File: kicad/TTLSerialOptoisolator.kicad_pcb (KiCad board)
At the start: 2 copper layers, 8 parts, among them P1 CONN_4, P2 CONN_4, U1 817C, U2 817C

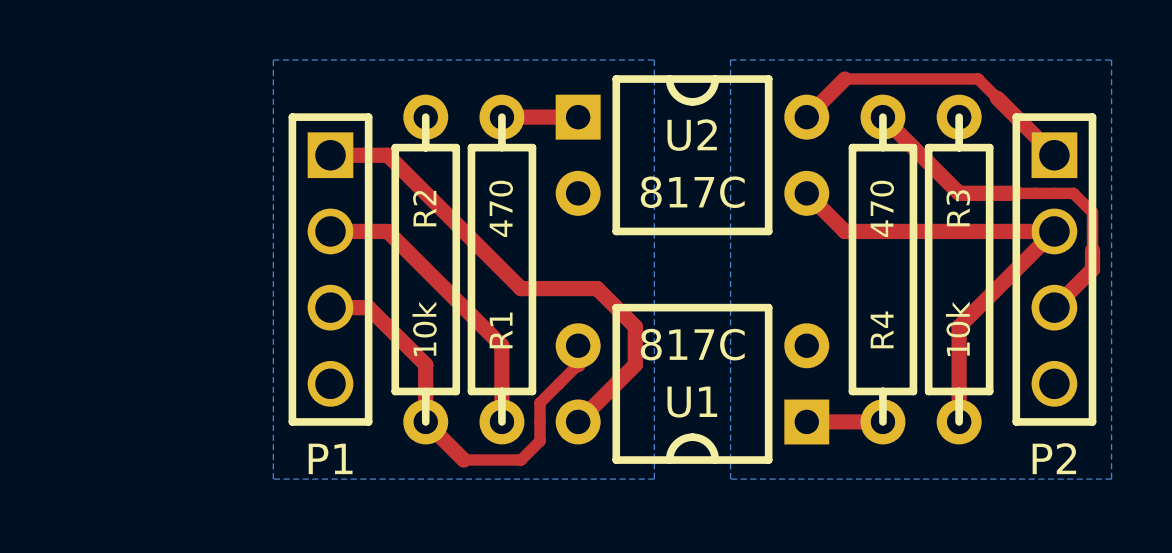
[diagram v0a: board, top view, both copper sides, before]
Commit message: iterating on board layout
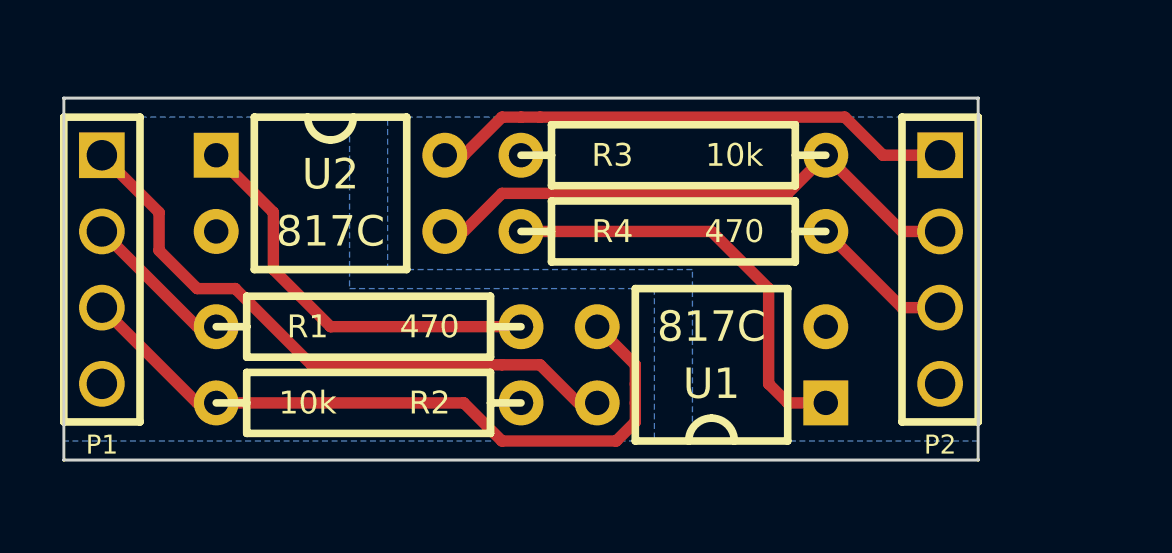
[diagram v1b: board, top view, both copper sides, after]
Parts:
- added G***: OSHW-logo_silkscreen-back_2mm, OSHW-logo_silkscreen-back_2mm, F.Cu at (139.1, 74.3)
- moved R3 14.7 mm to (146.7, 66.0), turned to 0 degrees
- moved R4 13.6 mm to (146.7, 68.6), turned to 0 degrees
- moved U2 12.1 mm to (140.3, 67.3)
- moved R1 10.0 mm to (136.5, 71.8), turned to 0 degrees
- moved R2 10.0 mm to (146.7, 74.3), turned to 180 degrees
- moved P1 7.62 mm to (132.7, 69.8)
- moved P2 3.81 mm to (160.7, 69.8)
- moved U1 0.90 mm to (153.0, 73.0)
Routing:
- net N-000003: track 2.54 -> 14.4 mm
- net N-0000010: track 2.54 -> 13.0 mm
- net RXa: track 14.2 -> 23.6 mm
- net 5Vb: track 9.83 -> 17.6 mm
- net TXb: track 12.0 -> 4.86 mm
- net TXa: track 9.83 -> 5.13 mm
- net 5Va: track 16.5 -> 20.0 mm
- net RXb: track 16.4 -> 18.0 mm
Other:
- board outline added: 30.5 x 12.1 mm
- board text added: "5V"
- board text added: "GND"
- board text added: "RX"
- board text added: "TTL Serial Optoisolator"
- board text added: "TX"
- board text added: "github.com/ pepaslabs/ TTLSerialOptoisolator"
- board text added: "v1"
